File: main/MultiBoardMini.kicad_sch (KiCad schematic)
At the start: 52 parts, among them J1 PB0, J2 PA10, J3 Conn_01x02_Male, J4 Conn_01x03, SW1 PF1, SW2 RESET, SW3 PF0, SW4 PF1, T1 PTS_1.5_2, T2 PTS_1.5_2, T3 PTS_1.5_2, U1 NUCLEO-F303K8, U3 M78AR5-1, U4 ESP32-C3-WROOM-02-N4

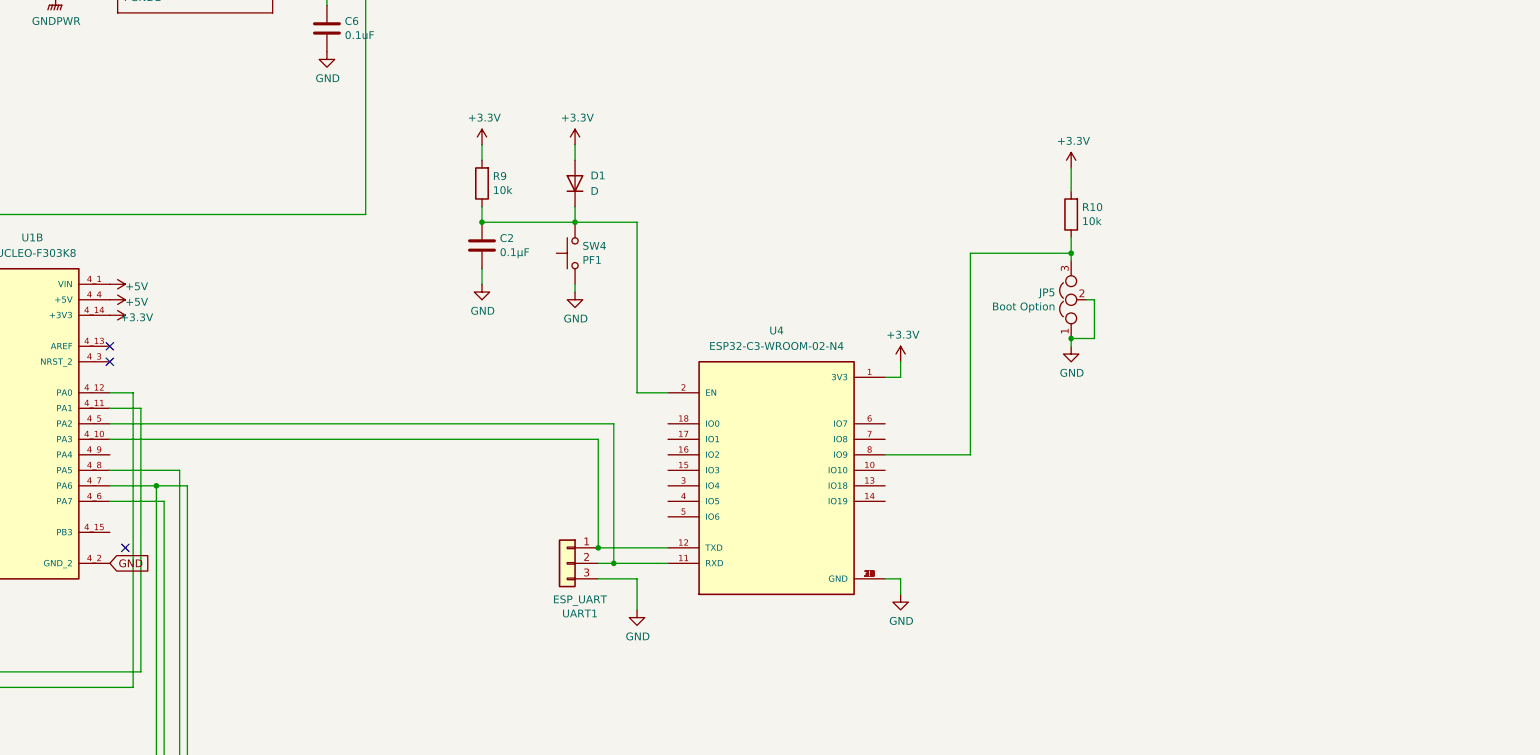
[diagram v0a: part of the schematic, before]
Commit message: 修正
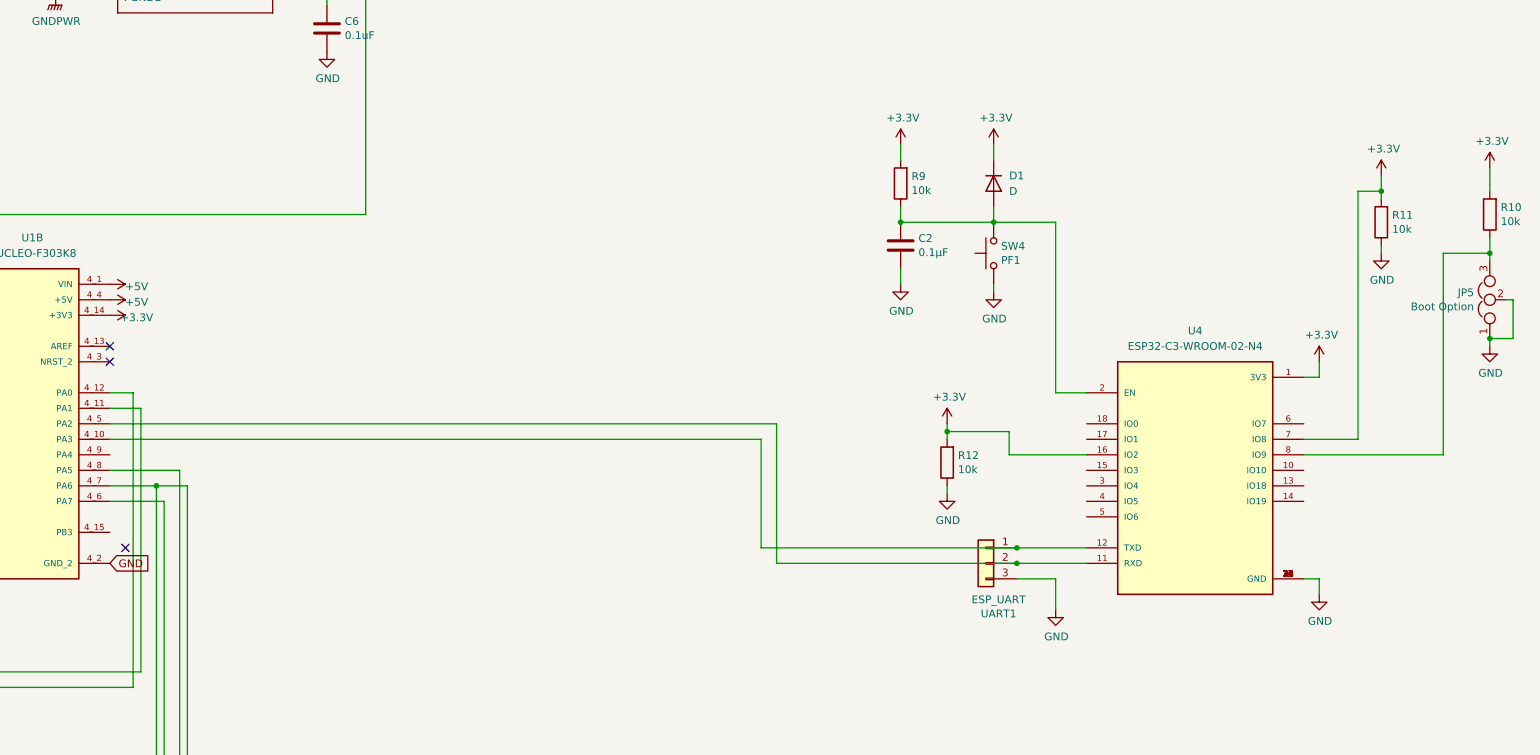
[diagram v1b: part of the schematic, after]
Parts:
- added R11, R12: 10k, Resistor_SMD:R_0603_1608Metric, symbol Device:R
- D1: footprint (none) -> Diode_SMD:D_SOD-123F
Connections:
- net +3V3: now also D1.1 (K), U4.16 (IO2), U4.7 (IO8), R11.2, R12.2; no longer D1.2 (A)
- net GND: now also R11.1, R12.1
- net at C2.1, R9.1, SW4.2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: now also D1.2 (A); no longer D1.1 (K)
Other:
- moved on the sheet: C2, D1, JP5, R10, R9, SW4, U4, UART1
